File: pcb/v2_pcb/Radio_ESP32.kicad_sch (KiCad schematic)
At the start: 16 parts, among them J800 ESP UART PROGRAM (pin 1 VTREF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, SW800 RESET, SW801 BOOT, U800 ESP32-C6-MINI-1

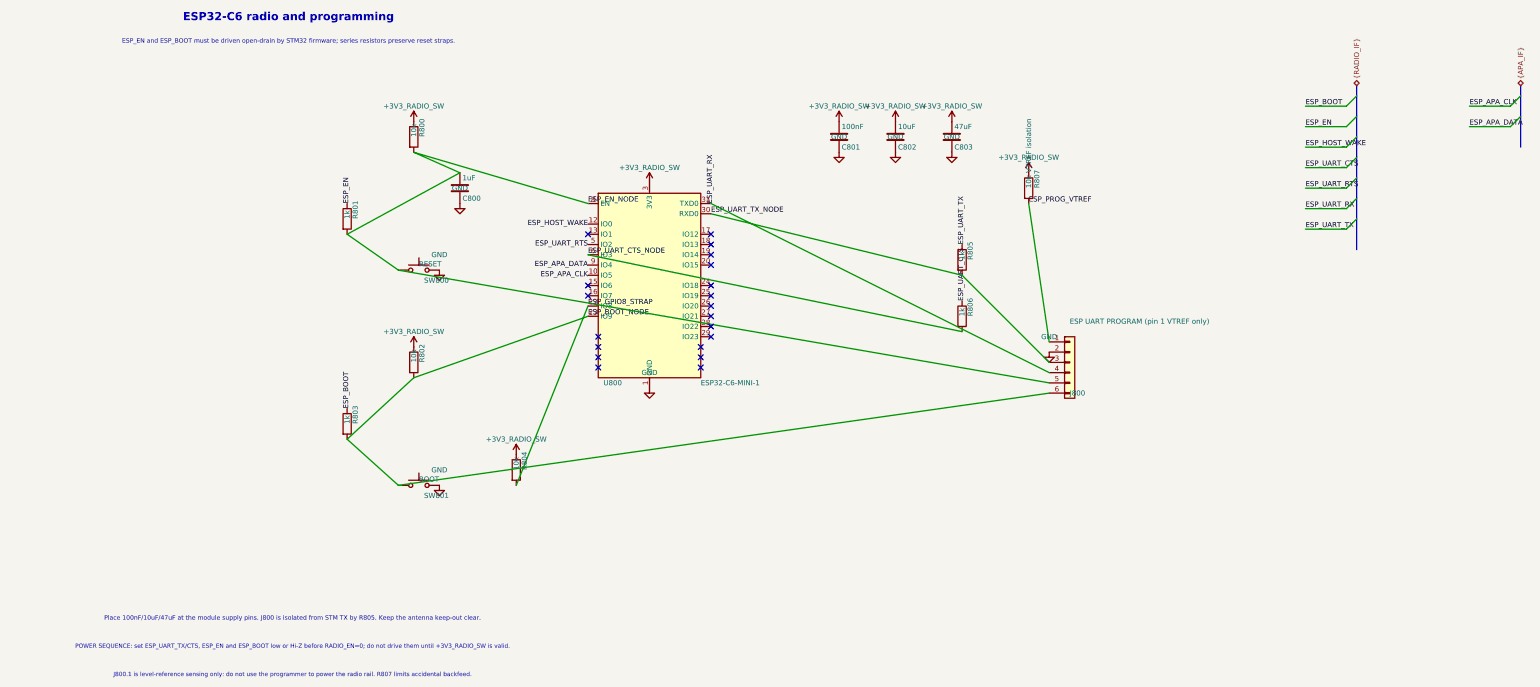
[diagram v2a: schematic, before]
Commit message: minor fixes
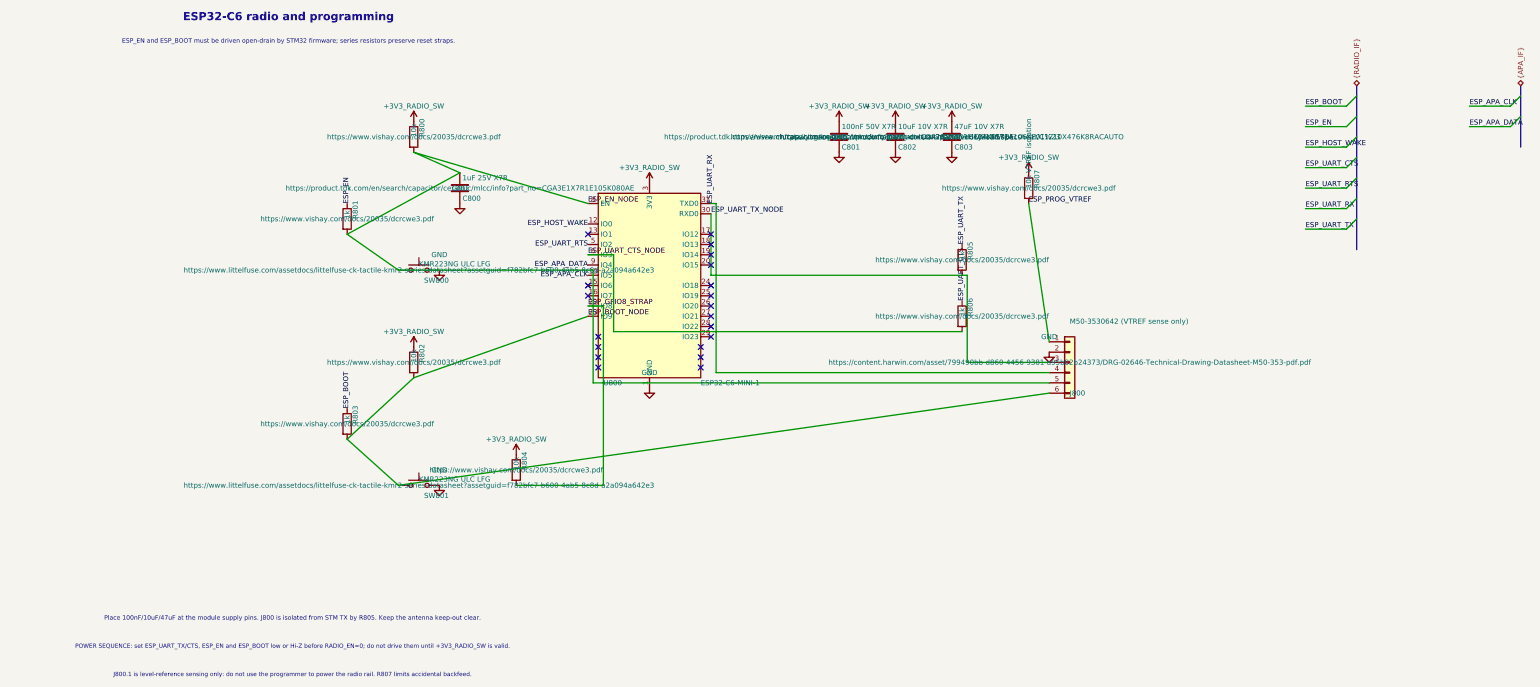
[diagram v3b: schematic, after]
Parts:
- C800: value 1uF -> 1uF 25V X7R; Dielectric (none) -> X7R; MPN (none) -> CGA3E1X7R1E105K080AE; Manufacturer (none) -> TDK; Qualification (none) -> AEC-Q200; Termination (none) -> Soft termination; Tolerance (none) -> ±10%; Voltage (none) -> 25 VDC
- C801: value 100nF -> 100nF 50V X7R; Dielectric (none) -> X7R; MPN (none) -> CGA2B3X7R1H104K050BE; Manufacturer (none) -> TDK; Qualification (none) -> AEC-Q200; Termination (none) -> Soft termination; Tolerance (none) -> ±10%; Voltage (none) -> 50 VDC
- C802: value 10uF -> 10uF 10V X7R; Dielectric (none) -> X7R; MPN (none) -> GCJ21BR71A106KE01L; Manufacturer (none) -> Murata; Qualification (none) -> AEC-Q200; Termination (none) -> Soft termination; Tolerance (none) -> ±10%; Voltage (none) -> 10 VDC
- C803: value 47uF -> 47uF 10V X7R; footprint Capacitor_SMD:C_0805_2012Metric -> Capacitor_SMD:C_1210_3225Metric; Dielectric (none) -> X7R; MPN (none) -> C1210X476K8RACAUTO; Manufacturer (none) -> KEMET (Yageo Group); Qualification (none) -> AEC-Q200; Release_Status (none) -> Verify effective capacitance under worst-case DC bias; Termination (none) -> FT-CAP flexible termination; Tolerance (none) -> ±10%; Voltage (none) -> 10 VDC
- J800: value ESP UART PROGRAM (pin 1 VTREF only) -> M50-3530642 (VTREF sense only); MPN (none) -> M50-3530642; Manufacturer (none) -> Harwin; Notes (none) -> Unpolarized 1x6 header; retain strong pin-1 mark; pin 1 VTR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
- R800, R802, R804, R807: MPN (none) -> CRCW040210K0FKED; Manufacturer (none) -> Vishay; Power (none) -> 0.063 W; TCR (none) -> ±100 ppm/K; Tolerance (none) -> ±1%
- R801, R803, R805, R806: MPN (none) -> CRCW04021K00FKED; Manufacturer (none) -> Vishay; Power (none) -> 0.063 W; TCR (none) -> ±100 ppm/K; Tolerance (none) -> ±1%
- SW800: value RESET -> KMR223NG ULC LFG; Contact (none) -> Gold ULC; 1 µA minimum at 1.8 V; MPN KMR221GLFS -> Y78B22324FP; Manufacturer C&K -> Littelfuse (C&K); Operating_Temperature (none) -> -40 to +125 °C
- SW801: value BOOT -> KMR223NG ULC LFG; Contact (none) -> Gold ULC; 1 µA minimum at 1.8 V; MPN KMR221GLFS -> Y78B22324FP; Manufacturer C&K -> Littelfuse (C&K); Operating_Temperature (none) -> -40 to +125 °C
